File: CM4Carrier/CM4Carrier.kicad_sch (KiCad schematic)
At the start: 0 parts

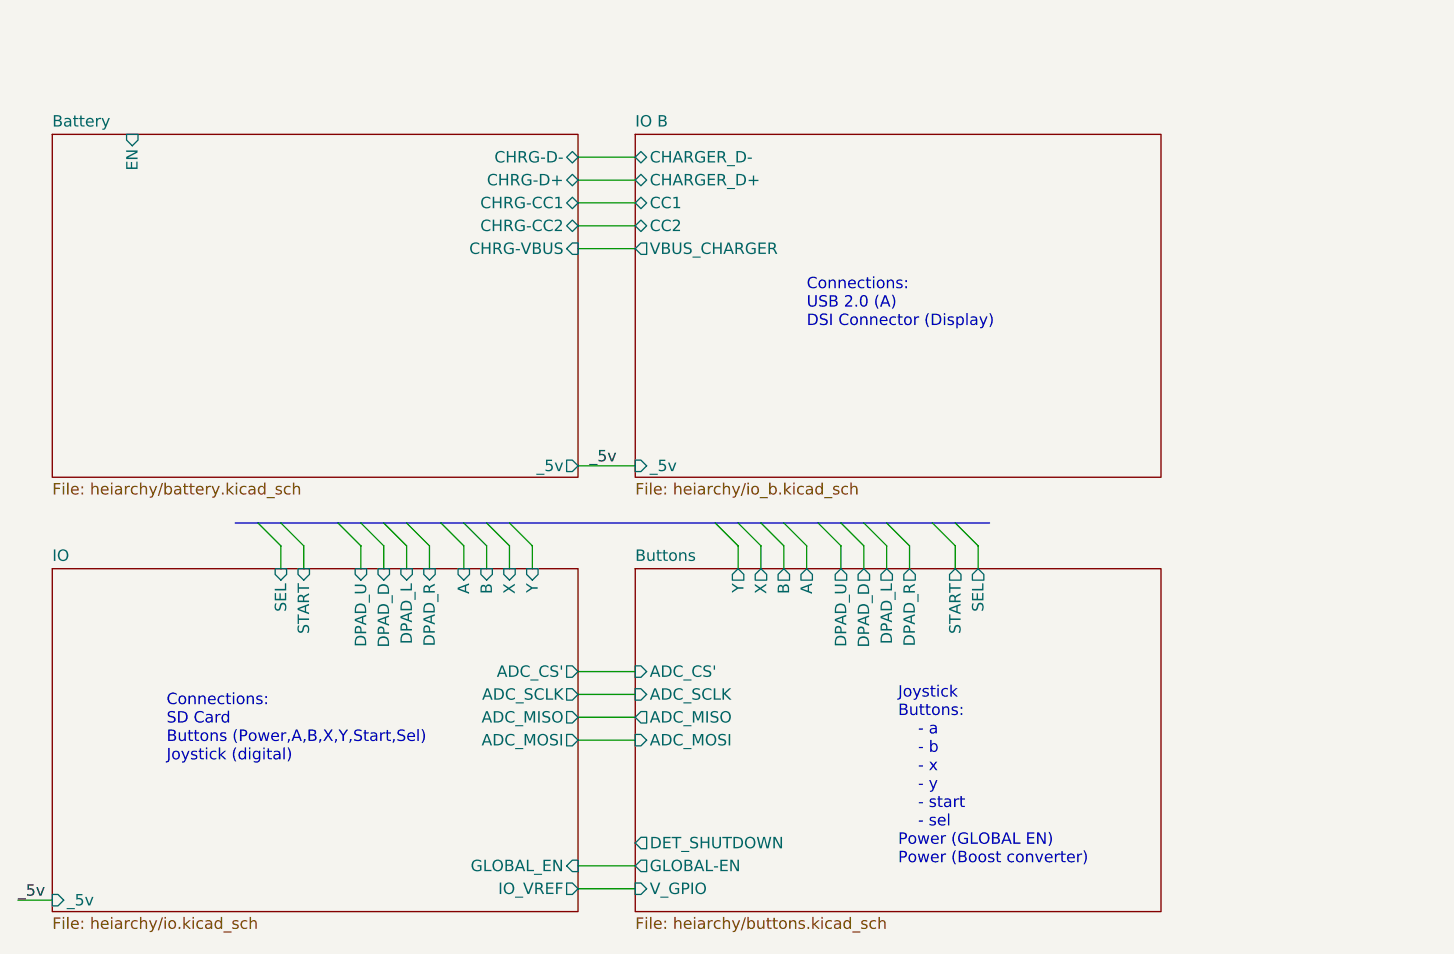
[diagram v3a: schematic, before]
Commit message: pcb babeee les goooo
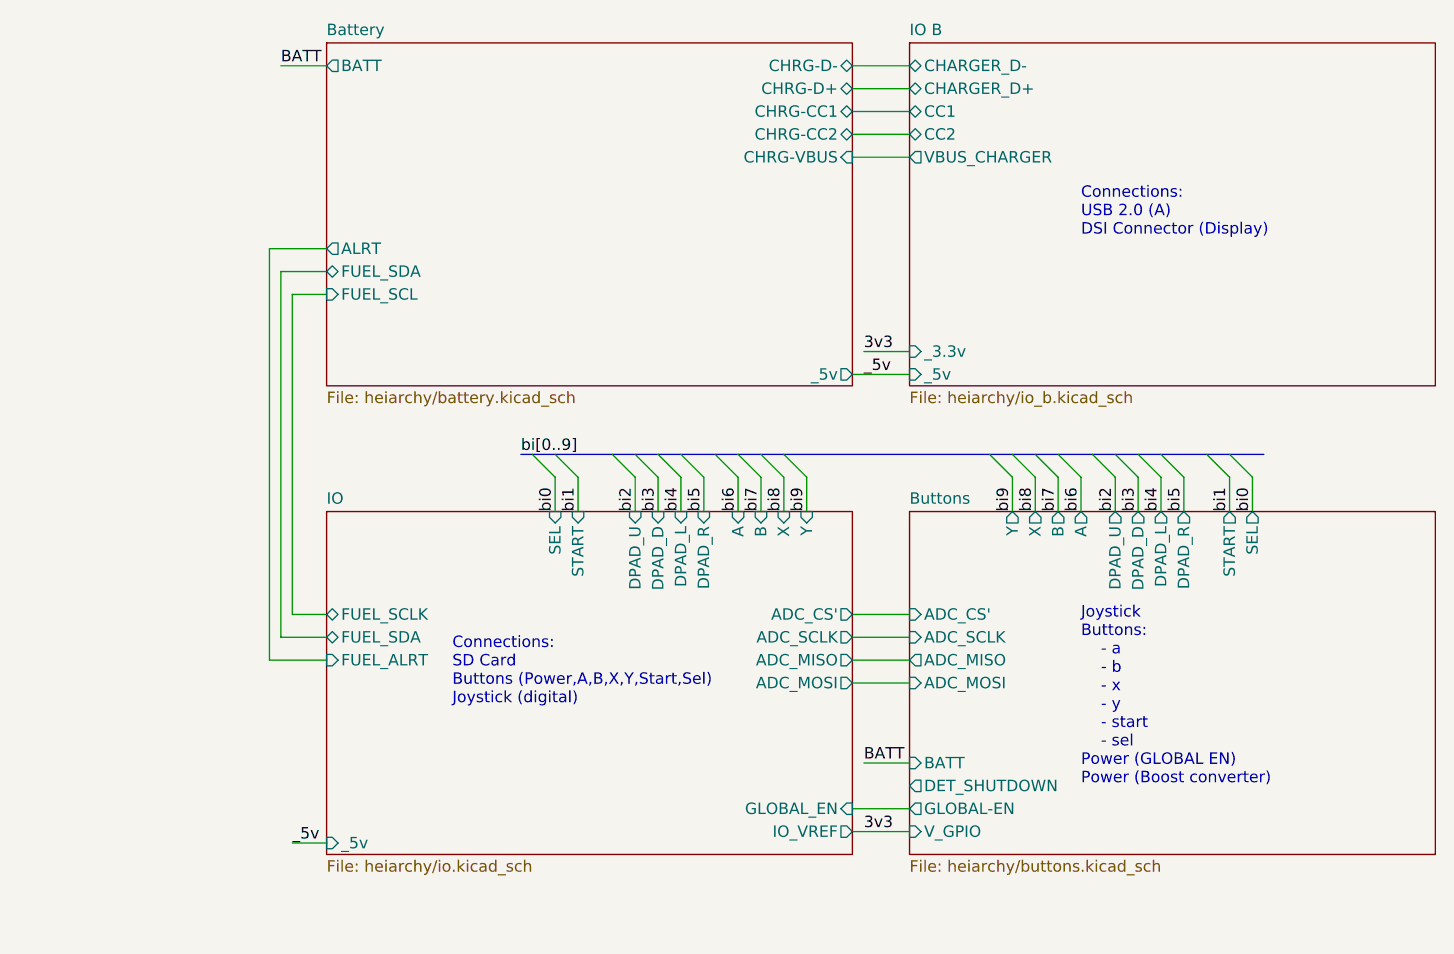
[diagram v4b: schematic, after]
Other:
- sheet Battery ports: added ALRT, BATT, FUEL_SCL, FUEL_SDA; removed EN
- sheet Buttons ports: added BATT; removed none
- sheet IO ports: added FUEL_ALRT, FUEL_SCLK, FUEL_SDA; removed none
- sheet IO B ports: added _3.3v; removed none
- title: (none) -> Cm4 battery carrier
